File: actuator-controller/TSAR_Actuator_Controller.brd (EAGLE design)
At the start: 151.1 x 154.9 mm, 143 parts, among them Q1 220mA/50V/3.5Ω, Q10 220mA/50V/3.5Ω, Q11 IRF9530, Q12 220mA/50V/3.5Ω, Q13 IRF9530, Q14 220mA/50V/3.5Ω, Q15 IRF9530, Q16 220mA/50V/3.5Ω, Q17 IRF9530, Q18 220mA/50V/3.5Ω, Q19 IRF9530, Q2 IRF9530, Q20 220mA/50V/3.5Ω, Q3 IRF9530, Q4 220mA/50V/3.5Ω, Q5 IRF9530, Q6 220mA/50V/3.5Ω, Q7 IRF9530, Q8 220mA/50V/3.5Ω, Q9 IRF9530

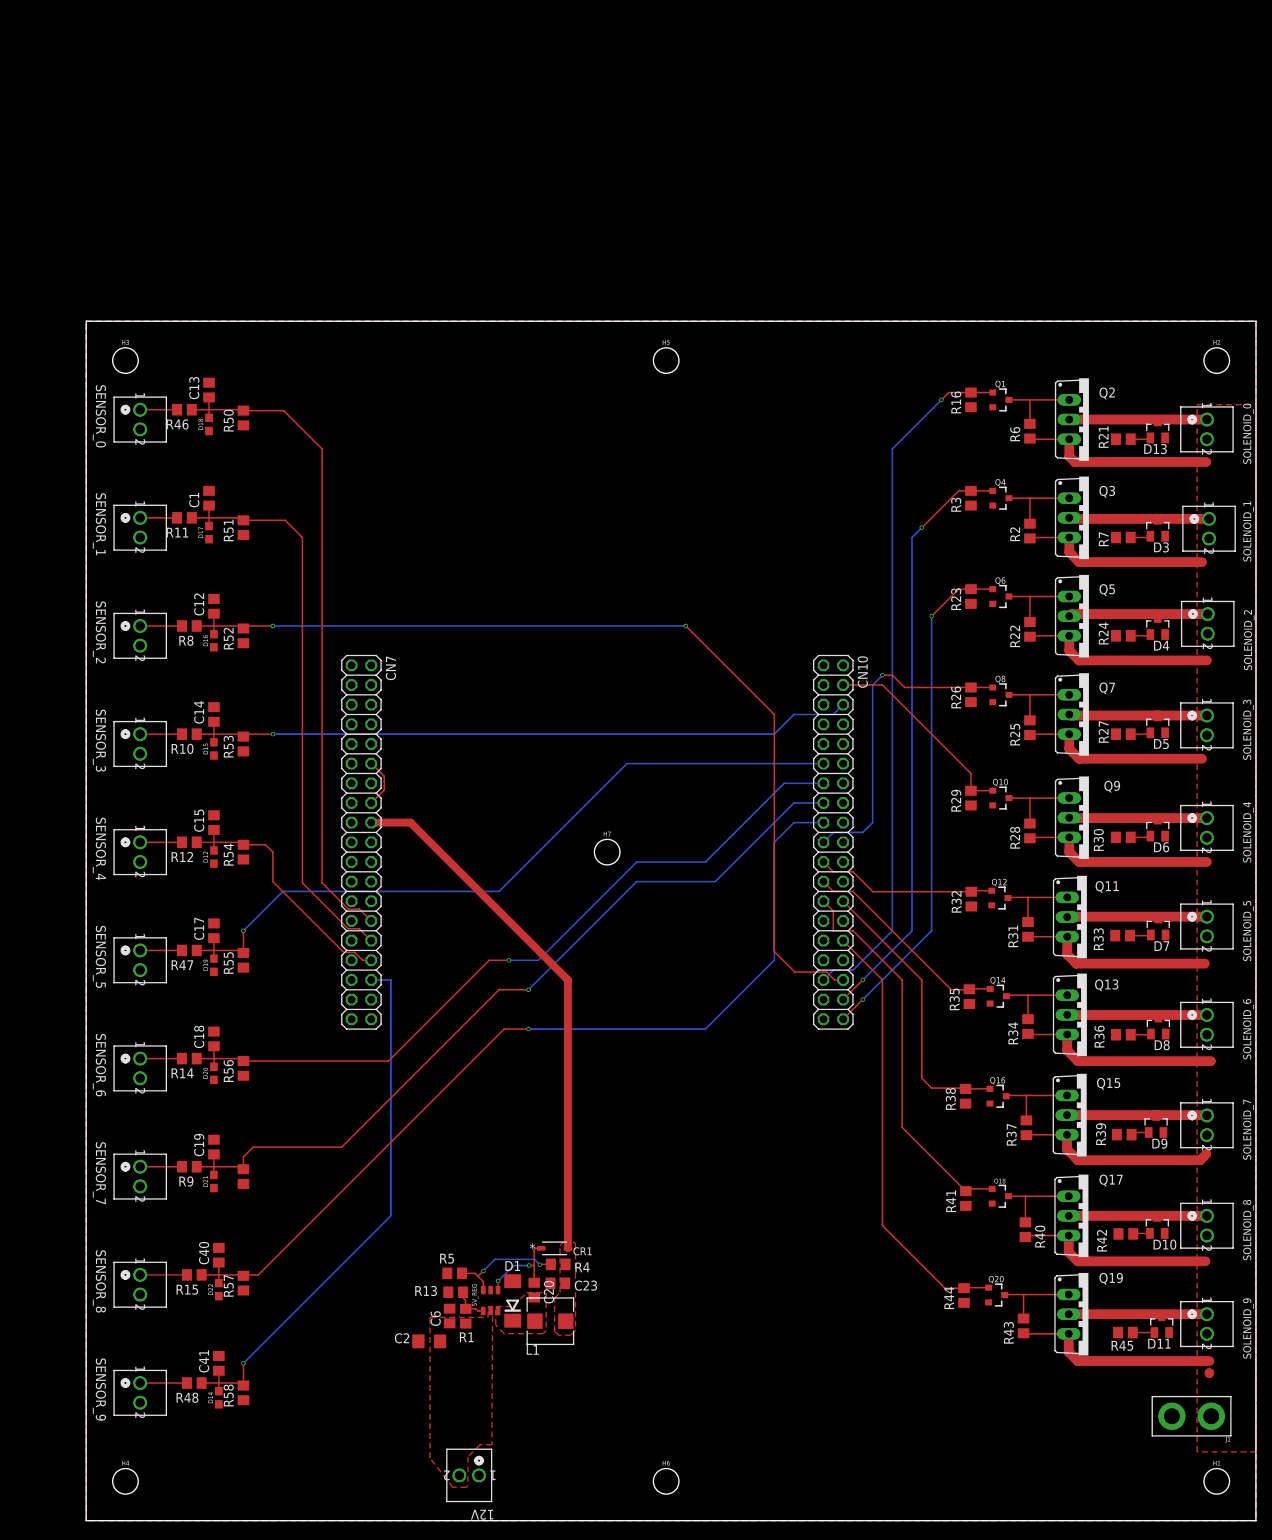
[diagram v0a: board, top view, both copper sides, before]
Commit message: Last Minute Fixes.
Corrected Morpho Connector Spacing.
Made all traces min 10 mil.
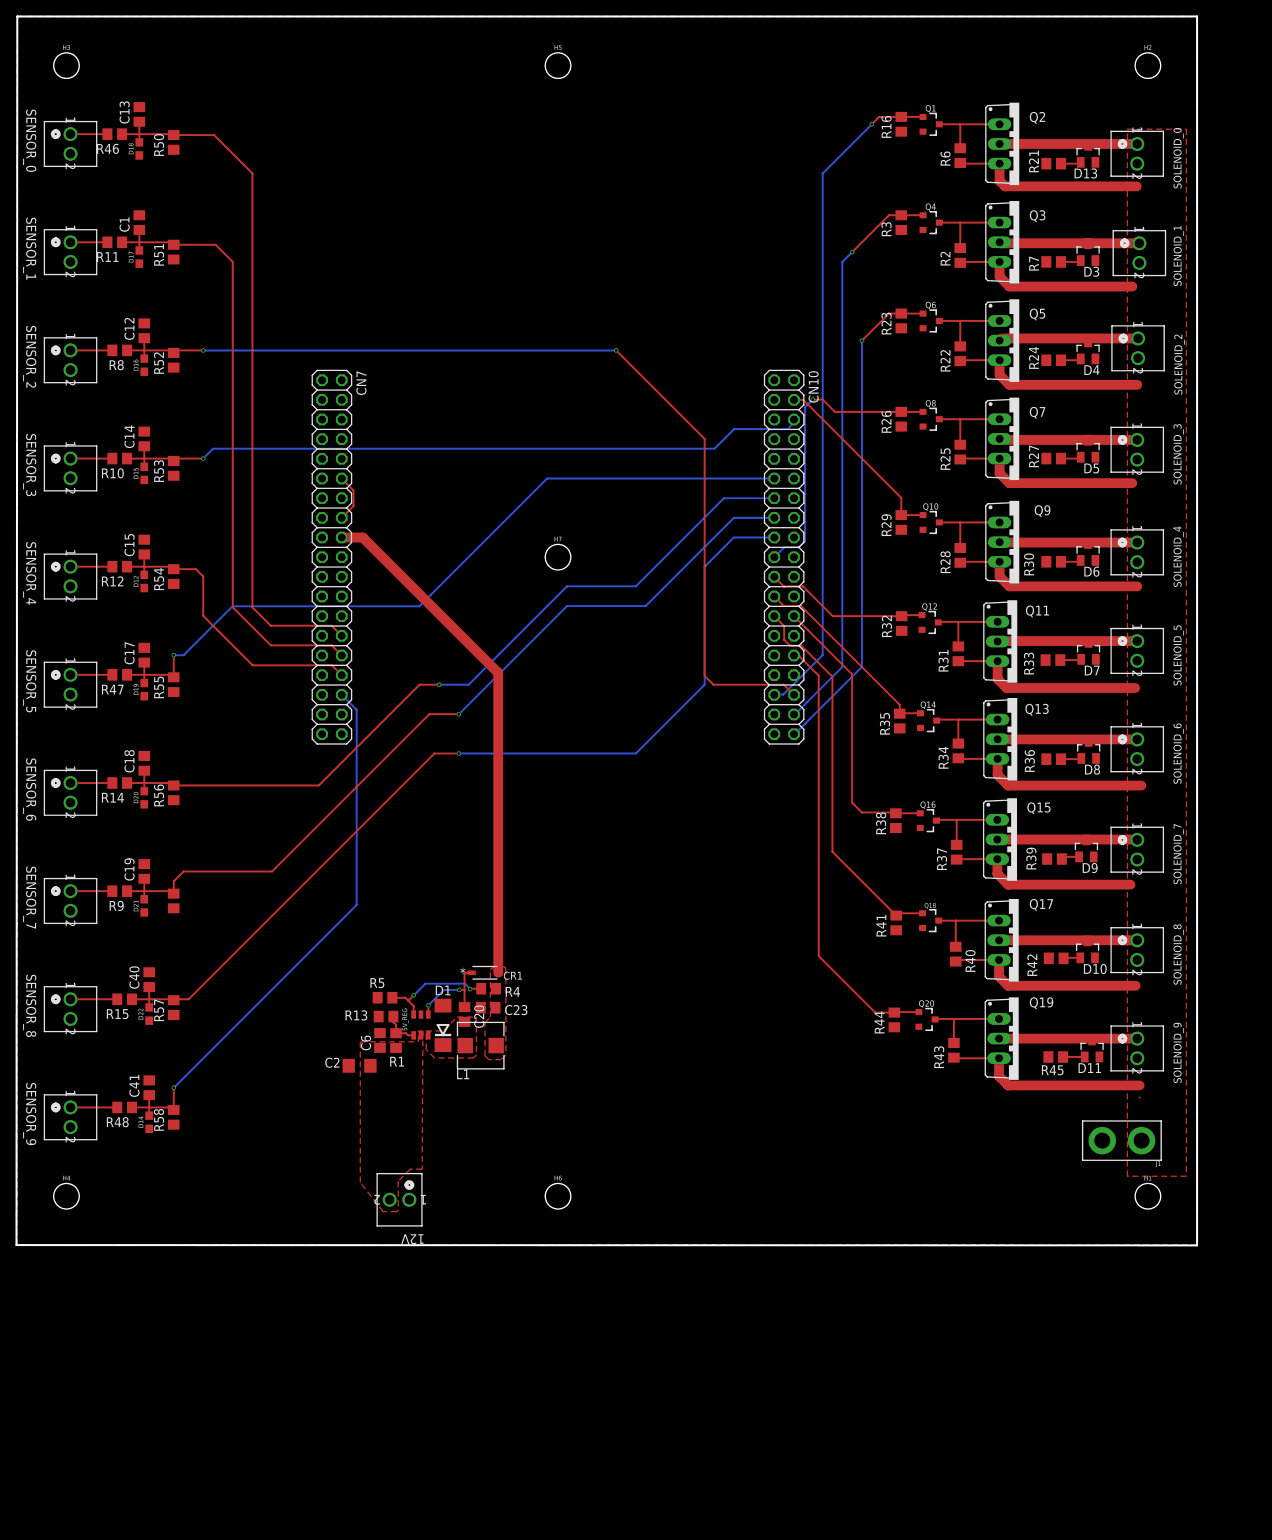
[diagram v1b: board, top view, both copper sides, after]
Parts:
- moved H5 40.6 mm to (69.8, 152.4)
- moved H6 39.4 mm to (69.8, 6.35)
- moved H2 39.1 mm to (146.1, 152.4)
- moved H3 38.9 mm to (6.35, 152.4)
- moved H7 38.6 mm to (69.8, 88.9)
- moved H1 37.9 mm to (146.1, 6.35)
- moved H4 37.6 mm to (6.35, 6.35)
- moved CN10 37.4 mm to (99.1, 88.9)
- moved CN7 37.0 mm to (40.6, 88.9)
- moved C1 36.7 mm to (15.8, 132.1)
- moved C12 36.7 mm to (16.4, 118.2)
- moved C13 36.7 mm to (15.8, 146.1)
- moved C14 36.7 mm to (16.4, 104.2)
- moved D18 36.7 mm to (15.8, 141.6)
- moved D3 36.7 mm to (138.3, 128.3)
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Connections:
- net AGND: no longer CN10.32
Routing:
- net TBD_SENSOR_4: track 33.7 -> 39.2 mm
- net TBD_SENSOR_1: track 74.6 -> 79.3 mm
- net TBD_SENSOR_0: track 86.0 -> 90.7 mm
- net SOL_GPIO_3: track 41.9 -> 38.4 mm
- net TBD_SENSOR_3: track 88.0 -> 91.4 mm
- net TBD_SENSOR_5: track 95.5 -> 98.7 mm
- net TBD_SENSOR_8: track 116.3 -> 119.4 mm
- net TBD_SENSOR_7: track 104.3 -> 107.5 mm
- net SOL_GPIO_0: track 89.7 -> 86.6 mm
- net TBD_SENSOR_6: track 98.6 -> 101.8 mm
- net +5V: track 68.5 -> 66.2 mm
- net SOL_GPIO_1: track 76.3 -> 74.1 mm, vias 2 -> 1
- net SOL_GPIO_2: track 66.1 -> 63.9 mm, vias 2 -> 1
- net SOL_GPIO_4: track 26.3 -> 24.1 mm
- net TBD_SENSOR_2: track 123.4 -> 125.6 mm
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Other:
- board size 151.1 x 154.9 mm -> 152.5 x 158.8 mm
